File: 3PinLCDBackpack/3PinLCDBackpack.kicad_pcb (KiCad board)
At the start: 2 copper layers, 54 x 19.7 mm, 7 parts, among them Q1 BC547, U1 74HC595, U2 LCD_HD44780, U3 5-pin_LiquidCrystal595_connec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

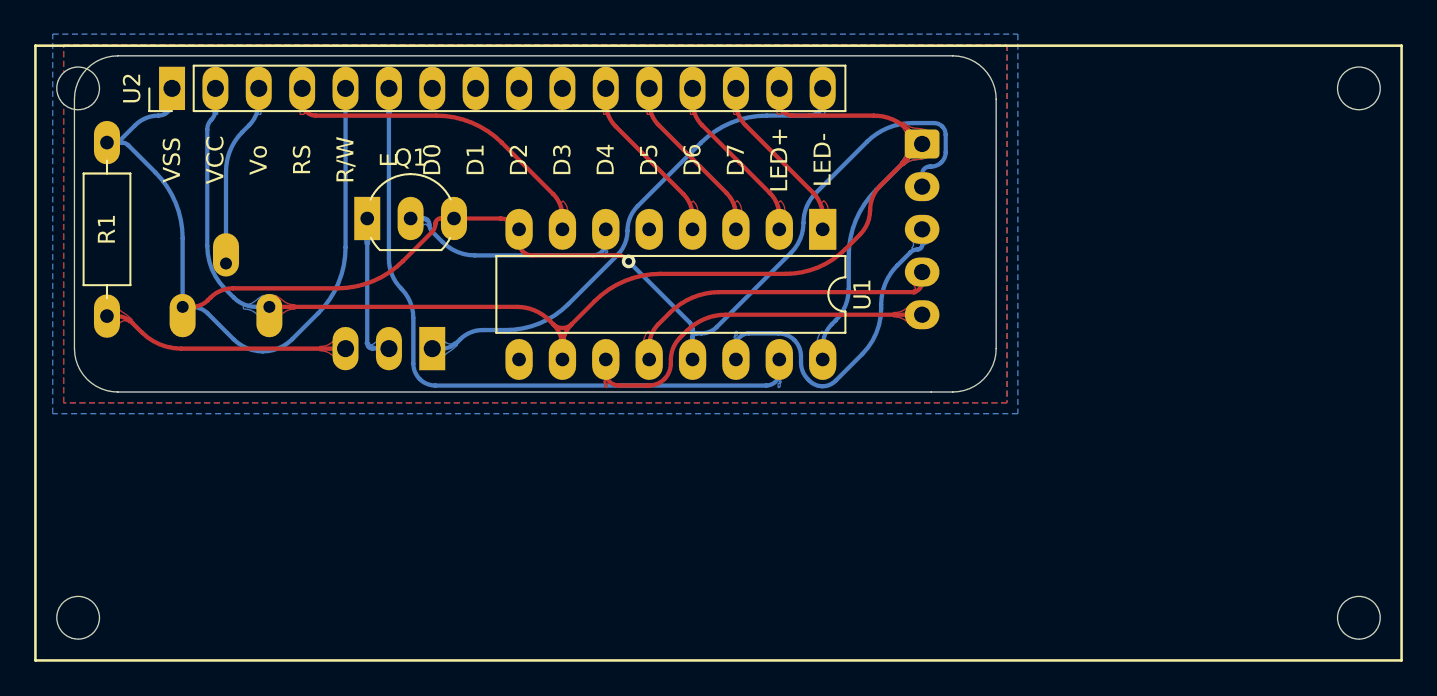
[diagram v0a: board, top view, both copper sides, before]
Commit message: 3-pin
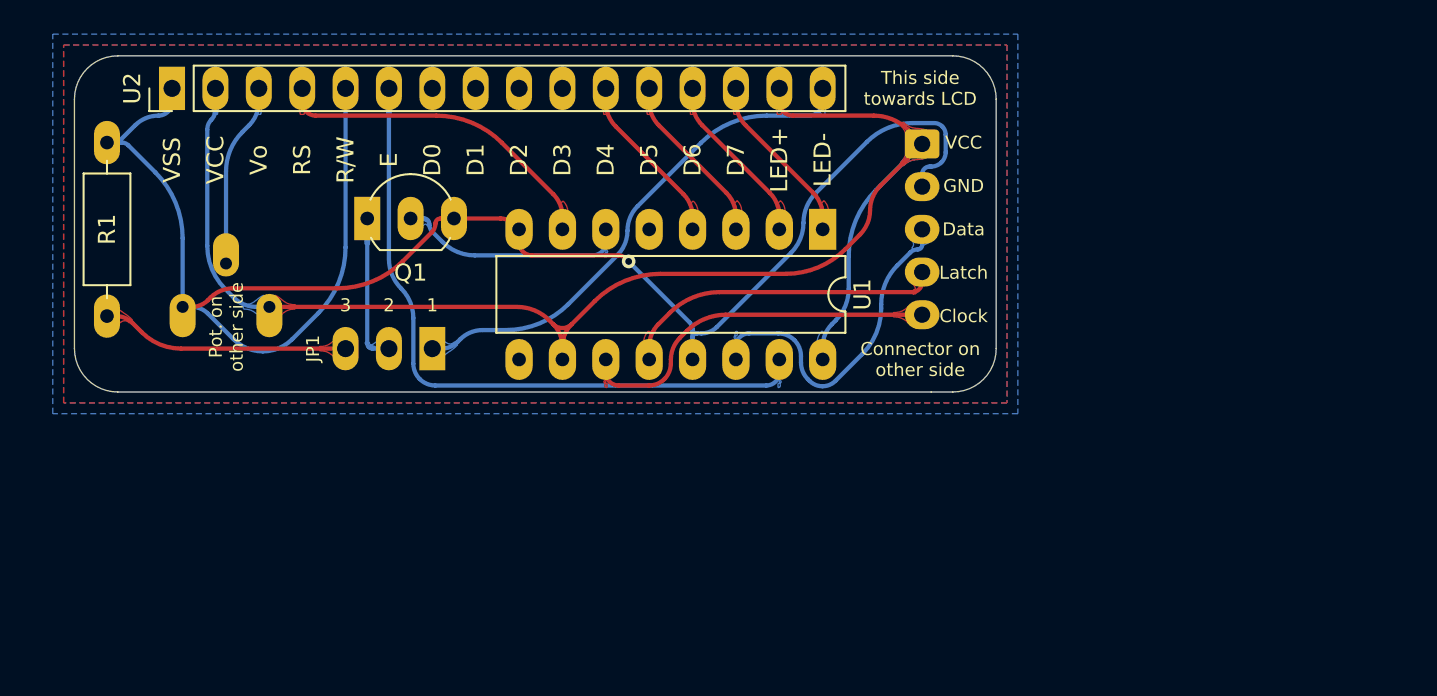
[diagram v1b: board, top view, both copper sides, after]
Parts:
- U2: footprint My_Parts:LCD_HD44780_16x2_w_headers_large -> My_Parts:LCD_HD44780_16x2_w_headers_no outlinelarge
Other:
- board text added: "1"
- board text added: "2"
- board text added: "3"
- board text added: "Clock"
- board text added: "Connector on other side"
- board text added: "Contrast"
- board text added: "Data"
- board text added: "GND"
- board text added: "JP1"
- board text added: "Latch"
- board text added: "Pot. on other side"
- board text added: "This side towards LCD"
- board text added: "VCC"
